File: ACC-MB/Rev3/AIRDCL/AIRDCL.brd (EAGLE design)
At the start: 172 x 64 mm, 20 parts, among them X13 5566-4

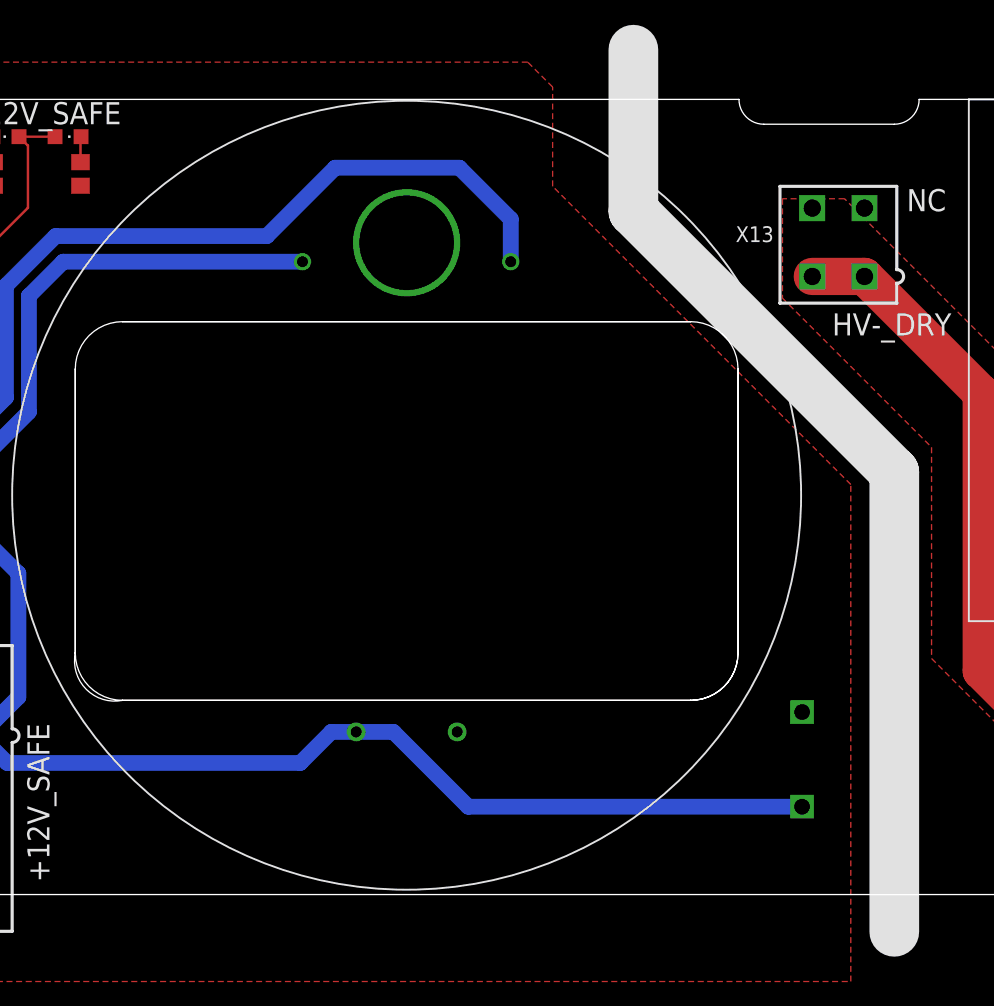
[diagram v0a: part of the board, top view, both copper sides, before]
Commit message: update
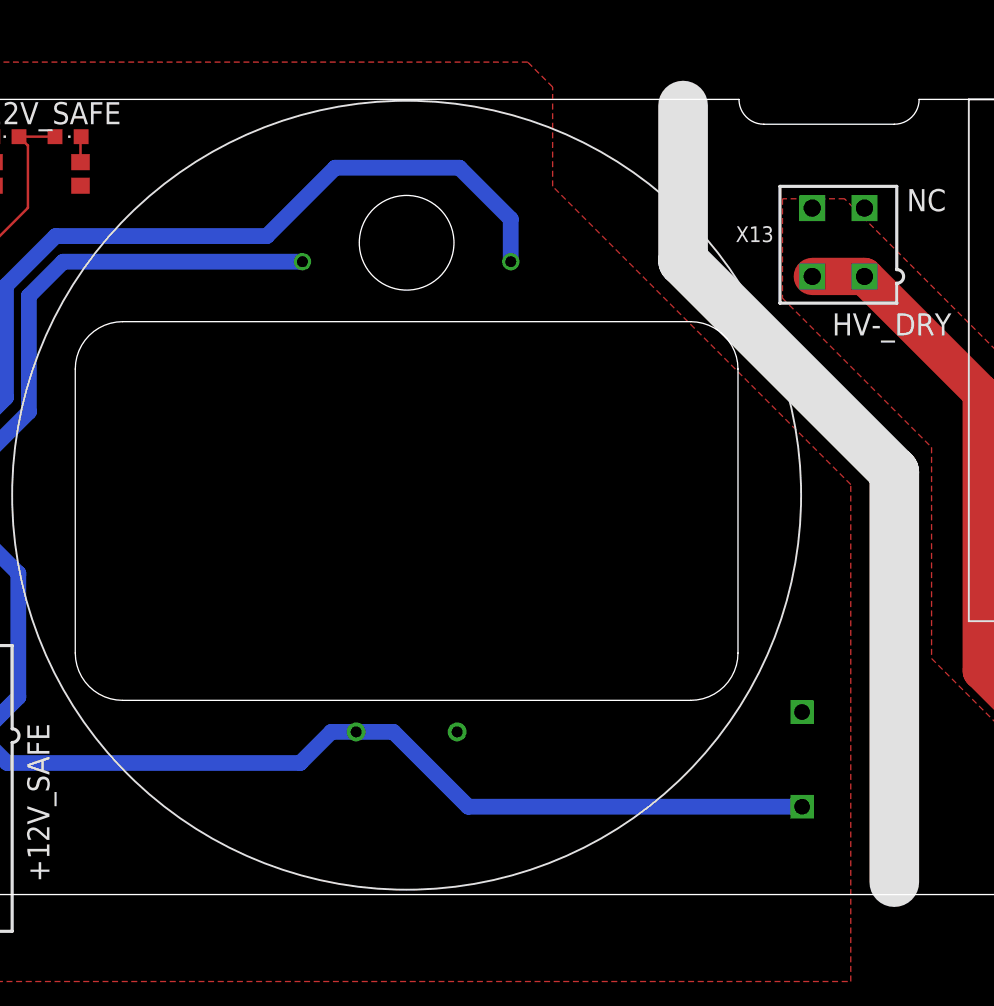
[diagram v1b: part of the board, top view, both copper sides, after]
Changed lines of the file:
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@@
 <layer number="42" name="bRestrict" color="1" fill="10" visible="yes" active="yes"/>
 <layer number="43" name="vRestrict" color="2" fill="10" visible="yes" active="yes"/>
-<layer number="44" name="Drills" color="7" fill="1" visible="no" active="yes"/>
-<layer number="45" name="Holes" color="7" fill="1" visible="no" active="yes"/>
-<layer number="46" name="Milling" color="3" fill="1" visible="no" active="yes"/>
-<layer number="47" name="Measures" color="7" fill="1" visible="no" active="yes"/>
+<layer number="44" name="Drills" color="7" fill="1" visible="yes" active="yes"/>
+<layer number="45" name="Holes" color="7" fill="1" visible="yes" active="yes"/>
+<layer number="46" name="Milling" color="3" fill="1" visible="yes" active="yes"/>
+<layer number="47" name="Measures" color="7" fill="1" visible="yes" active="yes"/>
 <layer number="48" name="Document" color="7" fill="1" visible="yes" active="yes"/>
 <layer number="49" name="Reference" color="7" fill="1" visible="yes" active="yes"/>
@@
 <wire x1="82.5" y1="62" x2="93" y2="62" width="0" layer="20"/>
 <wire x1="93" y1="62" x2="95" y2="64" width="0" layer="20" curve="90"/>
-<wire x1="72" y1="68" x2="72" y2="55" width="4" layer="21"/>
-<wire x1="72" y1="55" x2="93" y2="34" width="4" layer="21"/>
-<wire x1="93" y1="34" x2="93" y2="-3" width="4" layer="21"/>
 <text x="144" y="40.5" size="1.778" layer="26" rot="MR0">AIR Negative and Discharge Board
 Discharge R = 2x 2200 Ohm</text>
+<wire x1="93" y1="1" x2="93" y2="34" width="4" layer="25"/>
+<wire x1="93" y1="34" x2="76" y2="51" width="4" layer="25"/>
+<wire x1="76" y1="51" x2="76" y2="63.5" width="4" layer="25"/>
+<wire x1="76" y1="63.5" x2="76" y2="51" width="4" layer="26"/>
+<wire x1="76" y1="51" x2="93" y2="34" width="4" layer="26"/>
+<wire x1="93" y1="34" x2="93" y2="1" width="4" layer="26"/>
 </plain>
 <attributes>
@@
 <vertex x="63.5" y="67"/>
 </polygon>
+<wire x1="57.814" y1="13.09" x2="85.58" y2="14.69" width="0" layer="19" extent="1-1"/>
+<wire x1="27.5" y1="57.05" x2="57.814" y2="13.09" width="0" layer="19" extent="1-1"/>
+<wire x1="20.5" y1="57.05" x2="27.5" y2="57.05" width="0" layer="19" extent="1-1"/>
+<wire x1="6.25" y1="42.5" x2="20.5" y2="57.05" width="0" layer="19" extent="1-1"/>
+<wire x1="2.6" y1="18.29" x2="6.25" y2="42.5" width="0" layer="19" extent="1-1"/>
+<wire x1="2.6" y1="12.79" x2="2.6" y2="18.29" width="0" layer="19" extent="1-1"/>
 </signal>
 <signal name="N$5">
